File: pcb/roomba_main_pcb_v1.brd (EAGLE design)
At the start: 37 x 40 mm, 14 parts, among them J1 J25MM

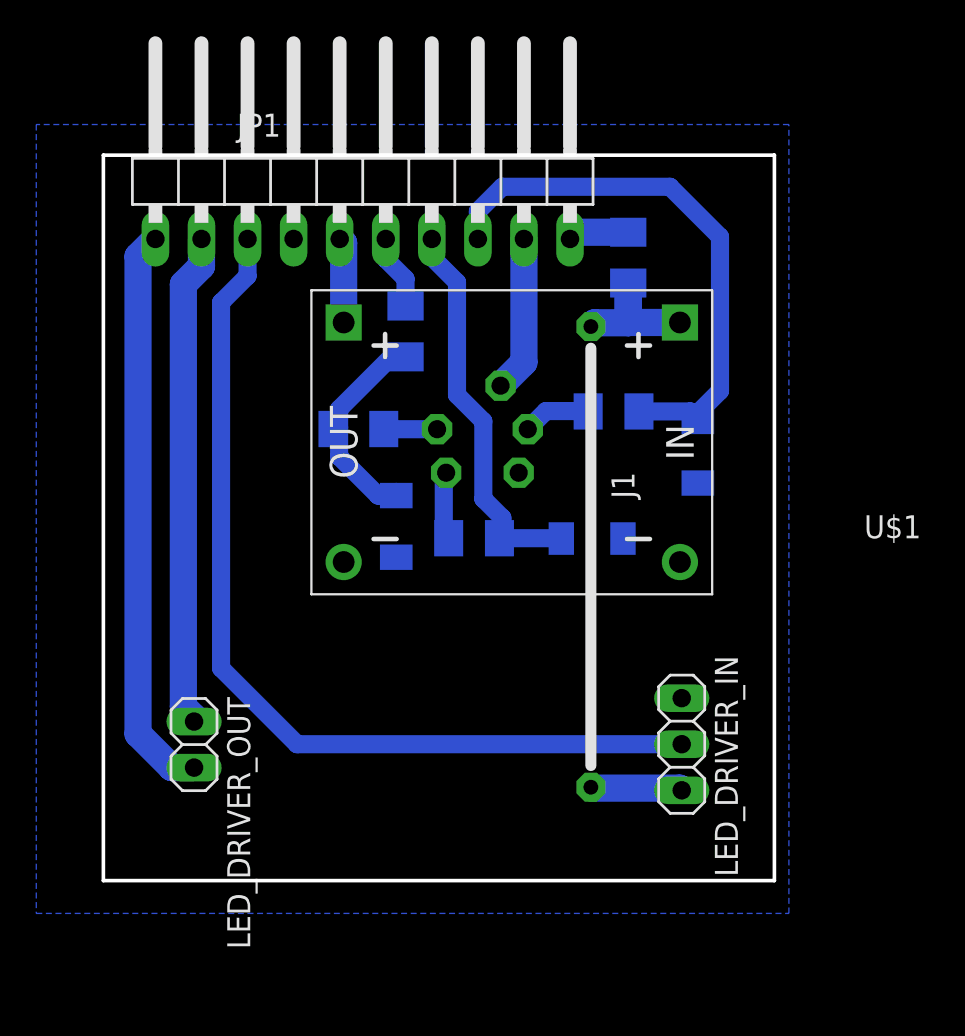
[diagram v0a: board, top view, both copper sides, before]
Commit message: 1.1
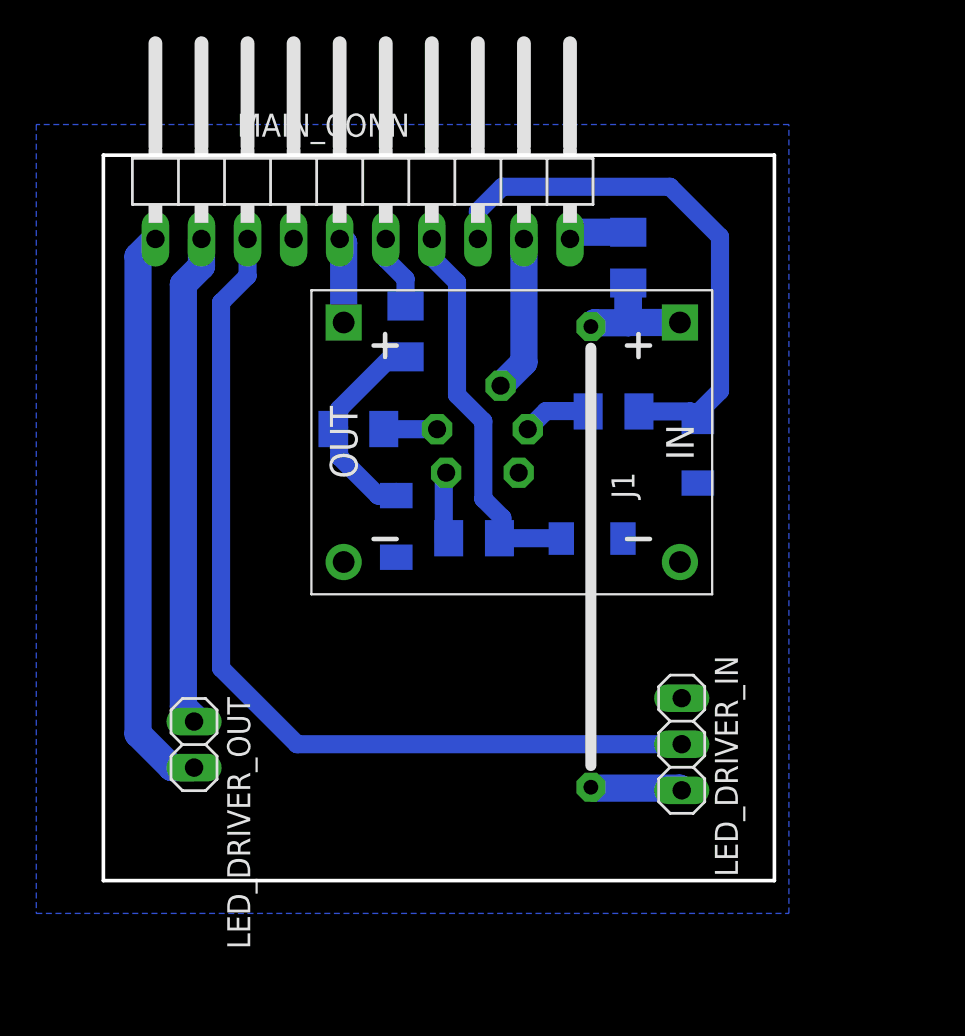
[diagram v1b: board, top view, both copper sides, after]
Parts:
- renumbered JP1 to MAIN_CONN
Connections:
- net 5V_RPI renamed RPI_5V
- net GND_LED renamed LED_GND
- net GPIO_14 renamed RPI_GPIO14
- net GPIO_15 renamed RPI_GPIO15
- net GPIO_18 renamed RPI_GPIO18
- net GPIO_23 renamed RPI_GPIO23
- net PWR_LED renamed LED_PWR
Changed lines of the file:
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@@
 <attribute name="VALUE" x="15.4" y="24.58" size="1.27" layer="28" rot="MR90"/>
 </element>
-<element name="JP1" library="pinhead" library_urn="urn:adsk.eagle:library:325" package="1X10/90" package3d_urn="urn:adsk.eagle:package:22408/2" value="" x="3.3" y="30.69" smashed="yes">
+<element name="MAIN_CONN" library="pinhead" library_urn="urn:adsk.eagle:library:325" package="1X10/90" package3d_urn="urn:adsk.eagle:package:22408/2" value="" x="3.3" y="30.69" smashed="yes">
 <attribute name="NAME" x="-3.6262" y="32.5188" size="1.27" layer="25" ratio="10"/>
 <attribute name="POPULARITY" value="1" x="3.3" y="30.69" size="1.778" layer="27" display="off"/>
@@
 </element>
 <element name="U$1" library="diy-modules" package="DC-DC-STEP-DOWN-MP1584" value="DC-DC-STEP-DOWN-MP1584" x="11.52" y="15.67" smashed="yes" rot="R180">
-<attribute name="NAME" x="32.52" y="11.645" size="1.27" layer="25" rot="R180" align="bottom-center"/>
 <attribute name="VALUE" x="32.02" y="12.195" size="1.27" layer="27" rot="R180" align="top-center"/>
 </element>
@@
 <contactref element="U$1" pad="IN-.1"/>
 <contactref element="LED_DRIVER_IN" pad="1"/>
-<contactref element="JP1" pad="4"/>
+<contactref element="MAIN_CONN" pad="4"/>
 </signal>
-<signal name="GPIO_15">
+<signal name="RPI_GPIO15">
 <contactref element="D2" pad="C"/>
 <contactref element="R2" pad="1"/>
@@
 <wire x1="21.78" y1="16.82" x2="21.78" y2="17.28" width="1" layer="16"/>
 <wire x1="21.78" y1="17.28" x2="23" y2="18.5" width="1" layer="16"/>
-<contactref element="JP1" pad="8"/>
+<contactref element="MAIN_CONN" pad="8"/>
 <wire x1="11" y1="29.757" x2="9.65" y2="28.407" width="1" layer="16"/>
 <wire x1="9.65" y1="28.407" x2="9.65" y2="26.88" width="1" layer="16"/>
@@
 <wire x1="2" y1="17.5" x2="2" y2="16.5" width="1" layer="16"/>
 </signal>
-<signal name="GPIO_23">
+<signal name="RPI_GPIO23">
 <contactref element="R4" pad="1"/>
 <contactref element="D3" pad="C"/>
@@
 <wire x1="8.5" y1="24.49" x2="7.11" y2="25.88" width="1" layer="16"/>
 <wire x1="7.11" y1="25.88" x2="7.11" y2="26.88" width="1" layer="16"/>
-<contactref element="JP1" pad="7"/>
+<contactref element="MAIN_CONN" pad="7"/>
 </signal>
 <signal name="N$4">
@@
 <signal name="+18V">
 <contactref element="ROOMBA_PORT" pad="VPWR_1"/>
-<contactref element="JP1" pad="9"/>
+<contactref element="MAIN_CONN" pad="9"/>
 <wire x1="12.19" y1="26.88" x2="12.19" y2="20.08" width="1.5" layer="16"/>
 <wire x1="12.19" y1="20.08" x2="10.9" y2="18.79" width="1.5" layer="16"/>
@@
 <wire x1="15.9" y1="17.39" x2="15.73" y2="17.37" width="0" layer="19" extent="16-16"/>
 </signal>
-<signal name="5V_RPI">
+<signal name="RPI_5V">
 <contactref element="U$1" pad="OUT+.2"/>
-<contactref element="JP1" pad="5"/>
+<contactref element="MAIN_CONN" pad="5"/>
 <wire x1="2.03" y1="26.88" x2="2.249" y2="26.661" width="1.5" layer="16"/>
 <wire x1="2.249" y1="26.661" x2="2.249" y2="22.274" width="1.5" layer="16"/>
@@
 <wire x1="17.94" y1="27.25" x2="14.98" y2="27.25" width="1.5" layer="16"/>
 <wire x1="14.98" y1="27.25" x2="14.92" y2="27.19" width="1.5" layer="16"/>
-<contactref element="JP1" pad="10"/>
+<contactref element="MAIN_CONN" pad="10"/>
 <wire x1="14.73" y1="26.88" x2="14.92" y2="27.19" width="0" layer="19" extent="16-16"/>
 </signal>
 <signal name="N$6">
-<contactref element="J1" pad="2"/>
 <contactref element="LED_DRIVER_IN" pad="3"/>
 <wire x1="20.77" y1="-3.4" x2="15.93" y2="-3.4" width="1.5" layer="16"/>
-<wire x1="15.88" y1="-3.35" x2="15.93" y2="-3.4" width="1.5" layer="16"/>
 <wire x1="20.89" y1="-3.52" x2="20.77" y2="-3.4" width="1.5" layer="16"/>
+<contactref element="J1" pad="2"/>
+<wire x1="15.88" y1="-3.35" x2="15.93" y2="-3.4" width="0" layer="19" extent="16-16"/>
 </signal>
-<signal name="GPIO_18">
+<signal name="RPI_GPIO18">
 <contactref element="LED_DRIVER_IN" pad="2"/>
 <wire x1="20.89" y1="-0.98" x2="-0.32" y2="-0.98" width="1" layer="16"/>
 <wire x1="-0.32" y1="-0.98" x2="-4.51" y2="3.21" width="1" layer="16"/>
-<contactref element="JP1" pad="3"/>
+<contactref element="MAIN_CONN" pad="3"/>
 <wire x1="-3.05" y1="26.88" x2="-3.05" y2="24.84" width="1" layer="16"/>
 <wire x1="-3.05" y1="24.84" x2="-4.51" y2="23.38" width="1" layer="16"/>
 <wire x1="-4.51" y1="23.38" x2="-4.51" y2="3.21" width="1" layer="16"/>
 </signal>
-<signal name="PWR_LED">
+<signal name="LED_PWR">
 <contactref element="LED_DRIVER_OUT" pad="2"/>
-<contactref element="JP1" pad="1"/>
+<contactref element="MAIN_CONN" pad="1"/>
 <wire x1="-9.09" y1="25.92" x2="-8.13" y2="26.88" width="1.5" layer="16"/>
 <wire x1="-6" y1="-2.27" x2="-7.23" y2="-2.27" width="1.5" layer="16"/>
@@
 <wire x1="-9.09" y1="-0.41" x2="-9.09" y2="25.92" width="1.5" layer="16"/>
 </signal>
-<signal name="GPIO_14">
-<contactref element="JP1" pad="6"/>
+<signal name="RPI_GPIO14">
+<contactref element="MAIN_CONN" pad="6"/>
 <contactref element="R1" pad="1"/>
 <wire x1="4.57" y1="26.88" x2="4.57" y2="25.77" width="1" layer="16"/>
@@
 <wire x1="5.66" y1="24.68" x2="5.66" y2="23.18" width="1" layer="16"/>
 </signal>
-<signal name="GND_LED">
+<signal name="LED_GND">
 <contactref element="LED_DRIVER_OUT" pad="1"/>
-<contactref element="JP1" pad="2"/>
+<contactref element="MAIN_CONN" pad="2"/>
 <wire x1="-5.59" y1="26.88" x2="-5.59" y2="25.38" width="1.5" layer="16"/>
 <wire x1="-5.59" y1="25.38" x2="-6.59" y2="24.38" width="1.5" layer="16"/>
